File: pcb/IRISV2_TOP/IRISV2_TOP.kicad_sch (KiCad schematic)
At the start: 13 parts, among them J1 Conn_01x20_MountingPin, J2 Conn_02x03_Odd_Even, J3 Conn_01x03, J4 Conn_01x02, J9 Conn_01x06_MountingPin

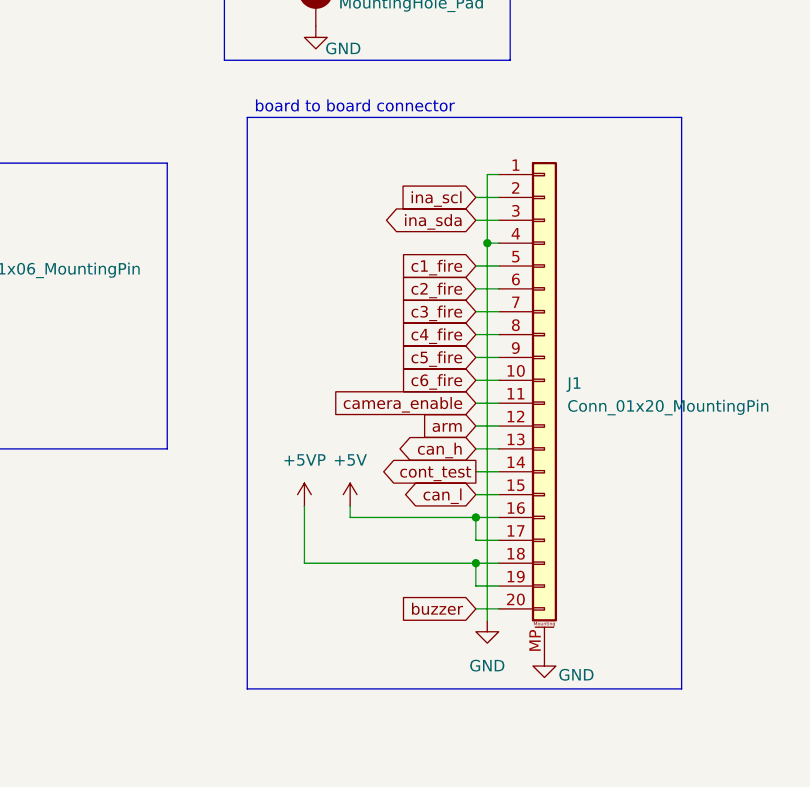
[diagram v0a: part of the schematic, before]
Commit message: pcb hopefully mostly finalized
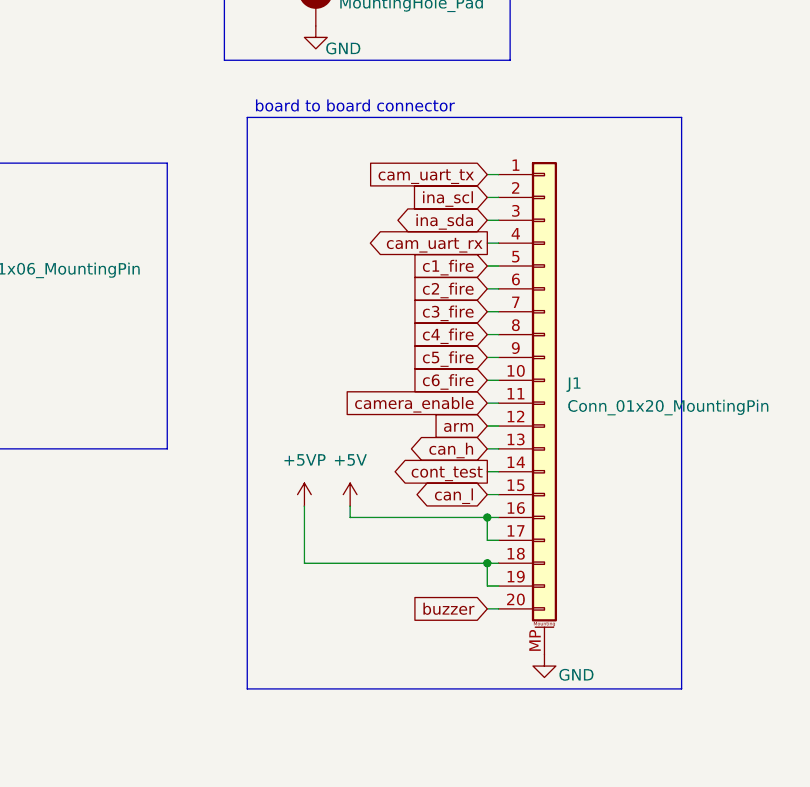
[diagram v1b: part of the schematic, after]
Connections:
- net GND: no longer J1.1 (Pin_1), J1.4 (Pin_4)
- new net cam_uart_rx: J1.4 (Pin_4)
- new net cam_uart_tx: J1.1 (Pin_1)
